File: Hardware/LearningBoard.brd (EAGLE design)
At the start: 68.8 x 83.5 mm, 54 parts, among them IC1 FT230XS-RFT230XS-R

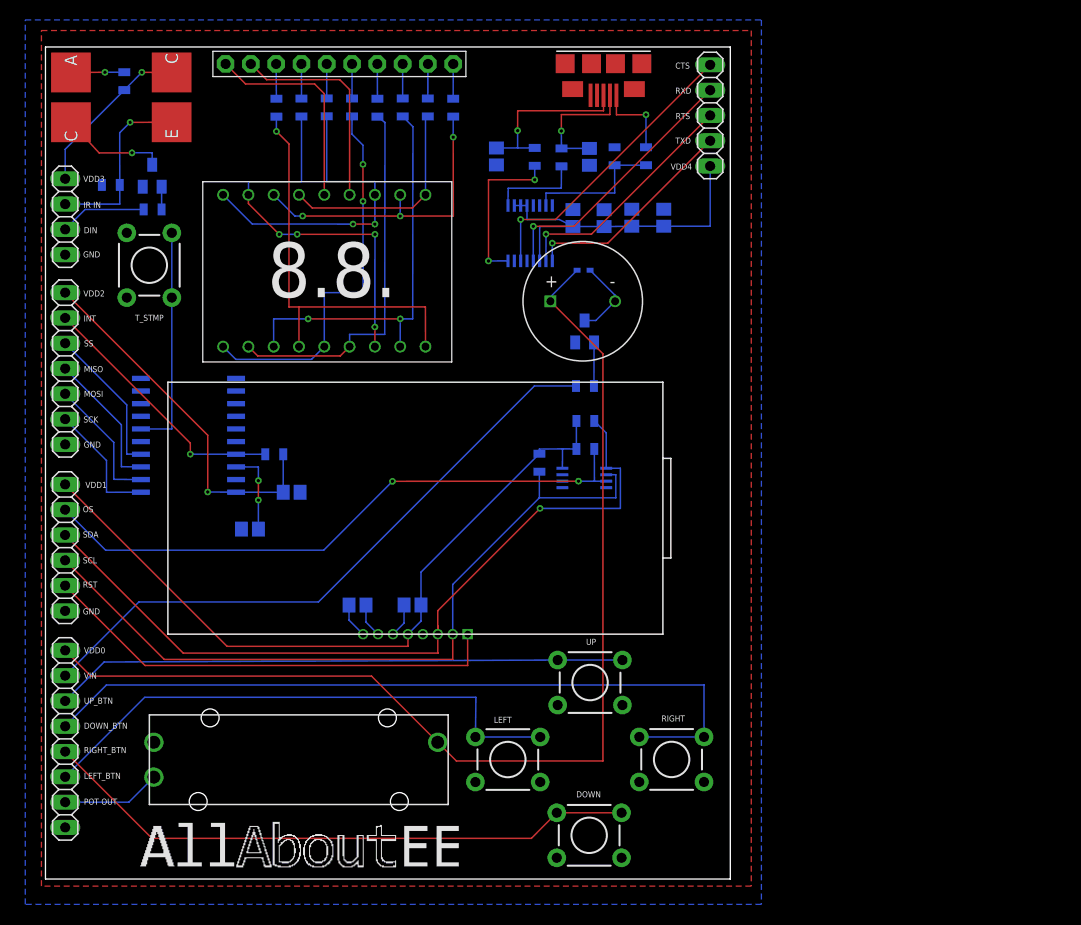
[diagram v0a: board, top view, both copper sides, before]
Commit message: New slim design.
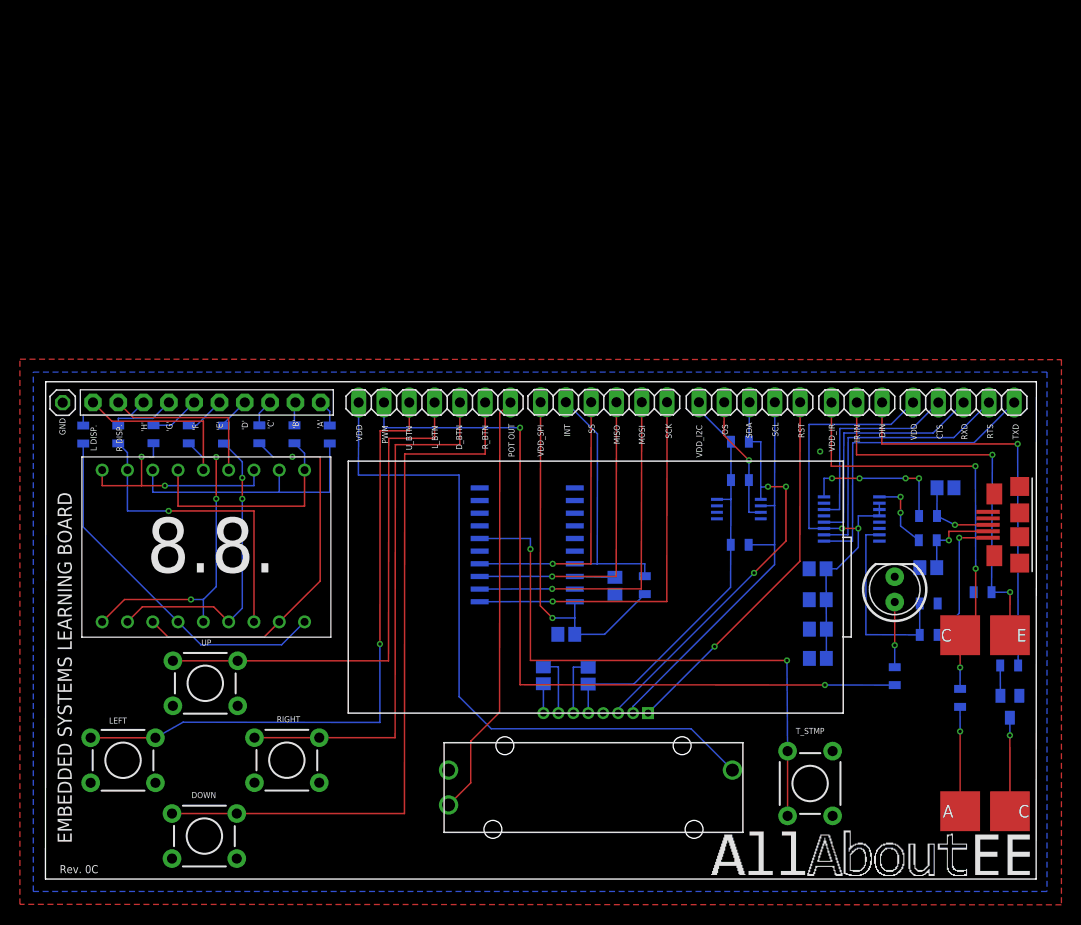
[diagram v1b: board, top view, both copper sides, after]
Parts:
- removed T2: (no value), transistor:SOT23-BEC
- removed U$8: 254-EMB-140-RO, AllAboutEE:254-EMB-140-RO
- removed U$9: 1N4148X-TP, AllAboutEE:SOD523
- added LED1: (no value), SparkFun-LED:LED5MM
- added VSS: VSS, pinhead:1X01
- D_A: device pinhead:1X08 -> pinhead:1X07
- I2C: device pinhead:1X06 -> pinhead:1X05
- R10: value 4k7 -> 4.7k
- R16: value 10k -> 510
- R17: value 10k -> 30
- R9: value 768 -> 1k
- SPI: device pinhead:1X07 -> pinhead:1X06
- TRANSMITTER: device pinhead:1X04 -> pinhead:1X03
- moved TRANSMITTER_ 116.4 mm to (94.3, 6.81), turned to 90 degrees
- moved R17 104.3 mm to (91.8, 18.2), turned to 90 degrees
- moved T1 101.3 mm to (96.8, 17.3), turned to 180 degrees
- moved RECEIVER_ 97.9 mm to (94.3, 24.5), turned to 270 degrees
- moved R16 97.4 mm to (96.8, 21.4), turned to 180 degrees
- moved R18 96.6 mm to (94.1, 28.8)
- moved T_STMP 84.3 mm to (76.8, 9.59), turned to 270 degrees
- moved TRANSMITTER 81.6 mm to (81.5, 47.8), turned to 180 degrees
- moved I2C 70.3 mm to (70.7, 47.9), turned to 180 degrees
- moved U$10 60.3 mm to (96.4, 35.6), turned to 90 degrees
- moved C6 56.0 mm to (90.4, 39.3), turned to 180 degrees
- moved R10 55.8 mm to (88.7, 24.5), turned to 0 degrees
- moved R11 54.9 mm to (88.7, 27.7), turned to 180 degrees
- moved SPI 54.2 mm to (56.1, 47.9), turned to 180 degrees
- moved R12 53.5 mm to (88.6, 36.4), turned to 0 degrees
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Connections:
- removed net N$29: R9.1, T2.B
- removed net VIN: D_A.7, R9.2
- new net PWM: D_A.6, R9.2
- net CTS: now also UART.4; no longer UART.1
- net DIN: now also TRANSMITTER.1; no longer TRANSMITTER.2
- net DOWN_BTN: now also D_A.2; no longer D_A.4
- net INT: now also SPI.5; no longer SPI.6
- net IR_RECEIVER: now also TRANSMITTER.2; no longer TRANSMITTER.3
- net LEFT_BTN: now also D_A.5; no longer D_A.3
- net MISO: now also SPI.3; no longer SPI.4
- net MOSI: now also SPI.2; no longer SPI.3
- net N$4: now also LED1.A, R9.1; no longer T2.C, U$8.NEGATIVE, U$9.A
- net OS: now also I2C.4; no longer I2C.5
- net POT_OUT: now also D_A.1; no longer D_A.2
- net RIGHT_BTN: now also D_A.3; no longer D_A.5
- net RST: now also I2C.1; no longer I2C.2
- net RTS: now also UART.2; no longer UART.3
- net RXD: now also UART.3; no longer UART.2
- net SCK: now also SPI.1; no longer SPI.2
- net SCL: now also I2C.2; no longer I2C.3
- net SDA: now also I2C.3; no longer I2C.4
- net SS: now also SPI.4; no longer SPI.5
- net TXD: now also UART.1; no longer UART.4
- net UP_BTN: now also D_A.4; no longer D_A.6
- net VDD: now also D_A.7; no longer D_A.8, U$8.POSITIVE, U$9.C
- net VDD_I2C: now also I2C.5; no longer I2C.6
- net VDD_IR: now also TRANSMITTER.3; no longer TRANSMITTER.4
- net VDD_SPI: now also SPI.6; no longer SPI.7
- net VSS: now also LED1.K, VSS.1; no longer D_A.1, I2C.1, SPI.1, T2.E, TRANSMITTER.1
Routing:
- net PWM: track 0.00 -> 79.6 mm, vias 0 -> 2
- net VIN: track 63.3 -> 0.00 mm
- net OS: track 62.1 -> 13.3 mm, vias 2 -> 1
- net VDD: track 111.2 -> 70.1 mm
- net SDA: track 80.7 -> 43.2 mm, vias 1 -> 3
- net N$27: track 22.8 -> 58.7 mm, vias 0 -> 2
- net SCL: track 76.5 -> 41.1 mm
- net POT_OUT: track 9.95 -> 43.0 mm
- net VDD_I2C: track 74.9 -> 42.6 mm
- net DIN: track 8.71 -> 40.0 mm, vias 0 -> 1
- net VDD_IR: track 16.9 -> 43.9 mm, vias 1 -> 3
- net SCK: track 12.5 -> 38.8 mm, vias 0 -> 1
- net RIGHT_BTN: track 77.6 -> 54.3 mm
- net MOSI: track 13.3 -> 35.0 mm, vias 0 -> 1
- net IR_RECEIVER: track 18.3 -> 38.9 mm, vias 1 -> 2
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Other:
- board size 68.8 x 83.5 mm -> 99.5 x 49.9 mm
- board text added: "'A'"
- board text added: "'B'"
- board text added: "'C'"
- board text added: "'D'"
- board text added: "'E'"
- board text added: "'F'"
- board text added: "'G'"
- board text added: "'H'"
- board text added: "D_BTN"
- board text added: "EMBEDDED SYSTEMS LEARNING BOARD"
- board text added: "L DISP."
- board text added: "L_BTN"
- board text added: "PWM"
- board text added: "R DISP."
- board text added: "R_BTN"
- board text added: "Rev. 0C"
- board text added: "U_BTN"
- board text added: "VDD"
- board text added: "VDD_I2C"
- board text added: "VDD_IR"
- board text added: "VDD_SPI"
- board text removed: "DOWN_BTN"
- board text removed: "LEFT_BTN"
- board text removed: "RIGHT_BTN"
- board text removed: "UP_BTN"
- board text removed: "VDD0"
- board text removed: "VDD1"
- board text removed: "VDD2"
- board text removed: "VDD3"
- board text removed: "VDD4"
- board text removed: "VIN"
